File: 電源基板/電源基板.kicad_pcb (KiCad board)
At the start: 2 copper layers, 59.7 x 49.5 mm, 24 parts, among them J1 XT30, J2 PWR out, J3 Power Switch, J4 5V out, J5 Conn_01x02_Pin, Q2 Q_NMOS_GDS, U1 OKL-T/6-W12N-C

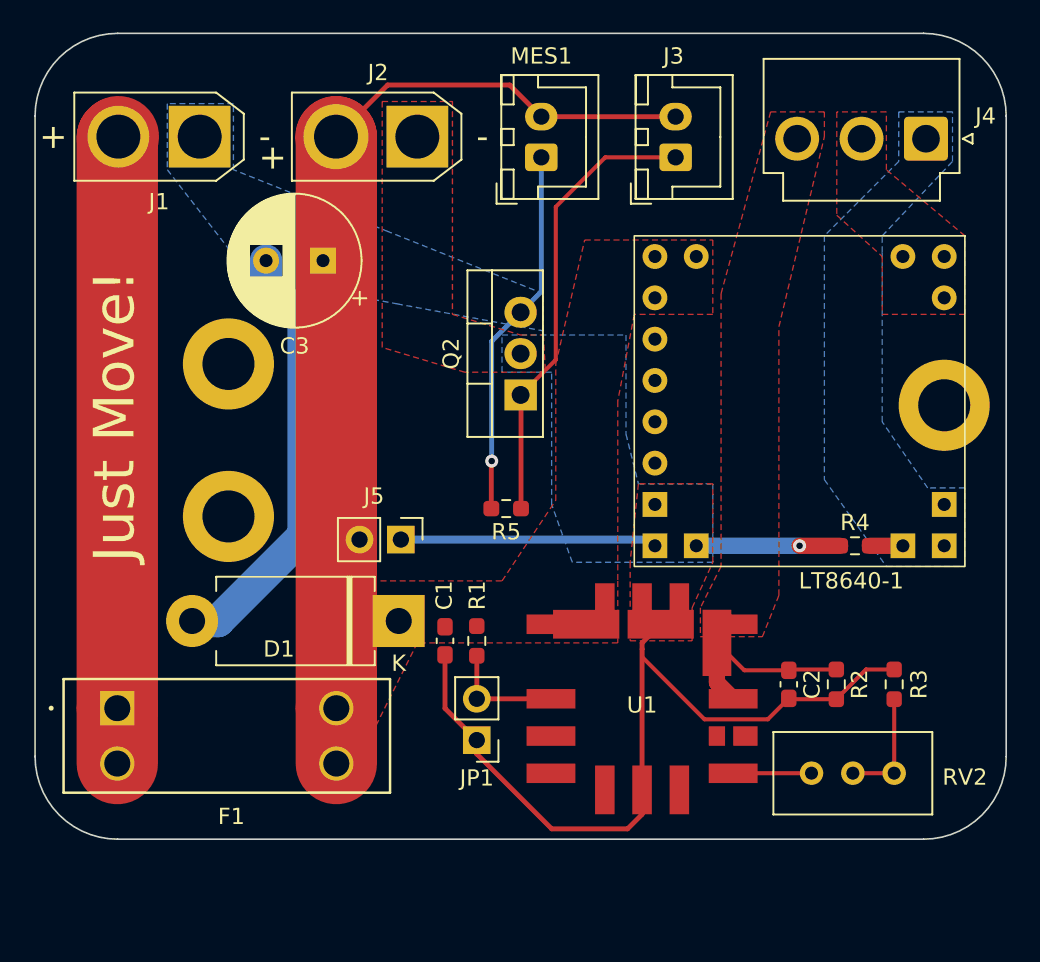
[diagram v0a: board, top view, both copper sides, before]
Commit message: 電源基板
白色にして発注
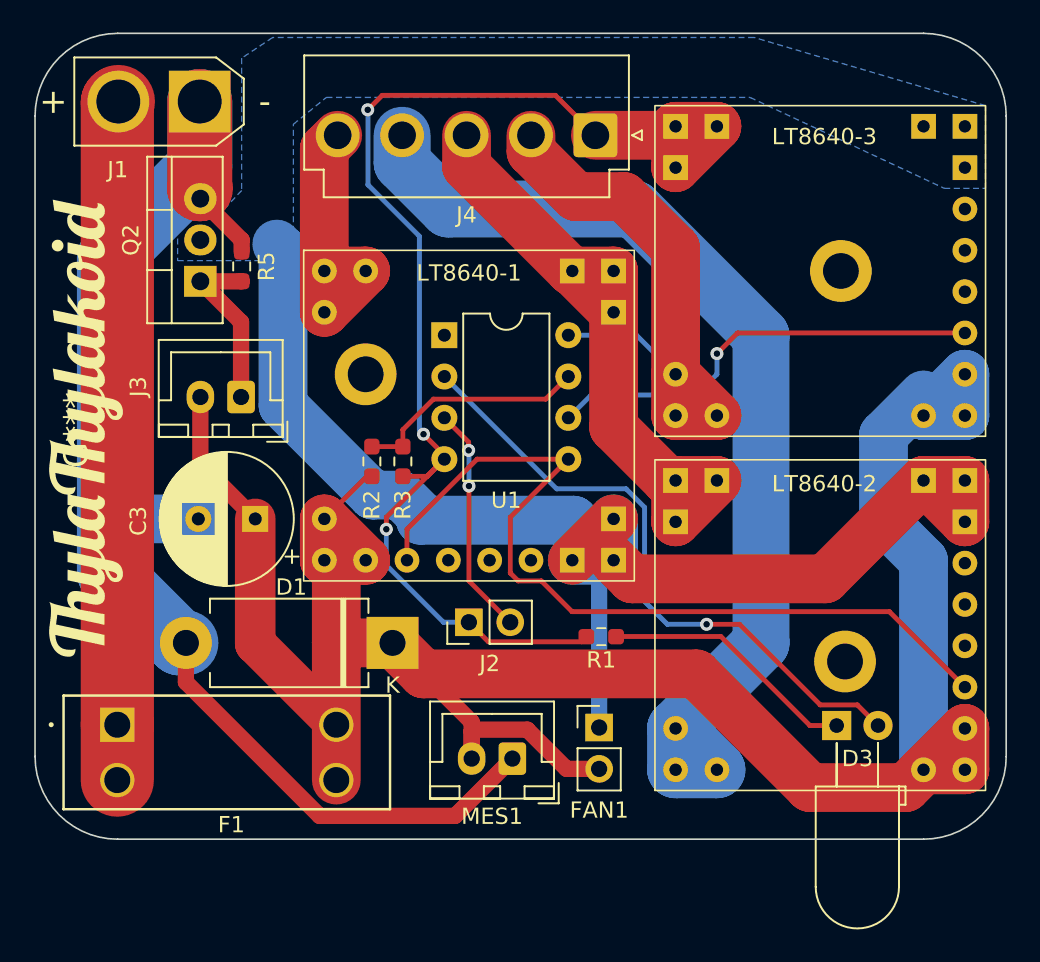
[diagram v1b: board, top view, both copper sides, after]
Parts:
- removed C1: 22u, Capacitor_SMD:C_0603_1608Metric_Pad1.08x0.95mm_HandSolder
- removed C2: 10u, Capacitor_SMD:C_0603_1608Metric_Pad1.08x0.95mm_HandSolder
- removed J5: Conn_01x02_Pin, Connector_PinHeader_2.54mm:PinHeader_1x02_P2.54mm_Vertical
- removed JP1: JumperShort, Connector_PinHeader_2.54mm:PinHeader_1x02_P2.54mm_Vertical
- removed R4: R_Small, Resistor_SMD:R_0603_1608Metric_Pad0.98x0.95mm_HandSolder
- removed the REF** at (42.4, 106.7)
- removed the REF** at (42.4, 116.1)
- removed the REF** at (86.4, 109.2)
- removed RV2: 20k, Potentiometer_THT:Potentiometer_Bourns_3296W_Vertical
- added D3: RED, LED_THT:LED_D5.0mm_Horizontal_O3.81mm_Z3.0mm, F.Cu at (79.8, 128.9)
- added FAN1: Conn_01x02_Pin, Connector_PinHeader_2.54mm:PinHeader_1x02_P2.54mm_Vertical, F.Cu at (65.2, 129.0)
- added G***: LOGO, logo:logo2, F.Cu at (33.0, 110.7)
- added LT8640-2: ~, LT8640:LT8640, F.Cu at (78.7, 122.7)
- added LT8640-3: ~, LT8640:LT8640, F.Cu at (78.7, 101.0)
- added REF**: MountingHole_2.2mm_M2_DIN965_Pad, MountingHole:MountingHole_2.2mm_M2_DIN965_Pad, F.Cu at (80.0, 101.0)
- added REF**: MountingHole_2.2mm_M2_DIN965_Pad, MountingHole:MountingHole_2.2mm_M2_DIN965_Pad, F.Cu at (80.3, 125.0)
- added REF**: MountingHole_2.2mm_M2_DIN965_Pad, MountingHole:MountingHole_2.2mm_M2_DIN965_Pad, F.Cu at (50.8, 107.3)
- J2: value PWR out -> Conn_01x02_Pin; footprint Connector_AMASS:AMASS_XT30U-F_1x02_P5.0mm_Vertical -> Connector_PinHeader_2.54mm:PinHeader_1x02_P2.54mm_Vertical
- J4: value 5V out -> PWR OUT; footprint Connector_JST:JST_VH_B3P-VH_1x03_P3.96mm_Vertical -> Connector_JST:JST_VH_B5P-VH_1x05_P3.96mm_Vertical
- R1: value 20k -> 220
- R2, R3: value 1.2k -> R_Small
- U1: value OKL-T/6-W12N-C -> ATtiny85-20P; footprint OKL-T_6-W12N-C:DCDC-murata-6A -> Package_DIP:DIP-8_W7.62mm
- moved MES1 37.0 mm to (59.8, 130.9), turned to 180 degrees
- moved R3 33.2 mm to (53.1, 112.7), turned to -90 degrees
- moved R2 31.7 mm to (51.2, 112.7), turned to 90 degrees
- moved J3 30.5 mm to (43.1, 108.7), turned to 180 degrees
- moved J2 30.0 mm to (57.1, 122.6), turned to 90 degrees
- moved U1 29.1 mm to (55.6, 104.9)
- moved R5 22.0 mm to (43.2, 100.7), turned to 90 degrees
- moved Q2 20.9 mm to (40.6, 101.6)
- moved LT8640-1 20.3 mm to (57.1, 109.9), turned to 180 degrees
- moved J4 20.3 mm to (64.9, 92.6)
- moved C3 16.4 mm to (44.0, 116.2)
- moved R1 7.65 mm to (65.3, 123.4), turned to 180 degrees
- moved J1 2.16 mm to (40.6, 90.6)
- moved D1 1.40 mm to (52.5, 123.8)
- moved F1 1.02 mm to (35.5, 128.9)
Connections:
- J2 pad 1: GND2 -> GND3
- J2 pad 2: VDD -> /tx
- J4 pad 1: GND2 -> GND3
- J4 pad 2: +5VA -> +5V
- J4 pad 3: +5VD -> GND1
- LT8640-1 pad 11: +5VA -> /6VA
- LT8640-1 pad 12: +5VA -> /6VA
- LT8640-1 pad 13: +5VA -> /6VA
- LT8640-1 pad 14: GND2 -> GND1
- LT8640-1 pad 15: GND2 -> GND1
- LT8640-1 pad 16: GND2 -> GND1
- LT8640-1 pad 4: unconnected-(LT8640-1-EN/UV-Pad4) -> /init_6v
- R1 pad 1: VDD -> Net-(D3-K)
- R1 pad 2: Net-(JP1-B) -> GND3
- R2 pad 1: +5VD -> VDD
- R2 pad 2: GND2 -> /Vref
- R3 pad 1: Net-(R3-Pad1) -> /Vref
- R3 pad 2: GND2 -> GND3
- U1 pad 1: Net-(JP1-B) -> unconnected-(U1-~{RESET}/PB5-Pad1)
- U1 pad 2: VDD -> /led
- U1 pad 3: GND2 -> /tx
- U1 pad 4: +5VD -> GND3
- U1 pad 5: +5VD -> /init_6v
- U1 pad 6: Net-(U1-TRIM1) -> /init_5v
- U1 pad 7: GND2 -> /Vref
- U1 pad 8: unconnected-(U1-NC-Pad8) -> +5V
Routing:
- net VDD: track 61.5 -> 152.4 mm
- net GND3: track 0.00 -> 78.0 mm, vias 0 -> 3
- net /6VB: track 0.00 -> 63.1 mm
- net /init_6v: track 0.00 -> 52.9 mm
- net GND1: track 0.00 -> 40.6 mm
- net /led: track 0.00 -> 38.9 mm, vias 0 -> 1
- net +5V: track 0.00 -> 36.4 mm
- net GND: track 49.7 -> 80.3 mm, vias 1 -> 0
- net /init_5v: track 0.00 -> 27.3 mm, vias 0 -> 1
- net Net-(J3-Pin_1): track 28.1 -> 10.7 mm
- net /6VA: track 0.00 -> 17.4 mm
- net Net-(D3-K): track 0.00 -> 15.8 mm
- net /Vref: track 0.00 -> 14.5 mm
- net /tx: track 0.00 -> 14.2 mm, vias 0 -> 2
- net +5VD: track 11.9 -> 0.00 mm
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- removed copper zone on F.Cu, net +5VA
- removed copper zone on F.Cu, net +5VD
- removed copper zone on B.Cu, net GND
- removed copper zone on F.Cu, net GND2
- removed copper zone on F.Cu, net VDD
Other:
- board text removed: "Just Move!"
